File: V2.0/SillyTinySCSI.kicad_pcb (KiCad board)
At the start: 4 copper layers, 53.5 x 25 mm, 48 parts, among them J1 DB25_Plug, J2 Micro_SD_Card_Det1, U1 74LVT125, U2 74LVT245, U3 74LVT125, U4 74LVT245, U5 TLV75728PDBVR, U6 Pico W

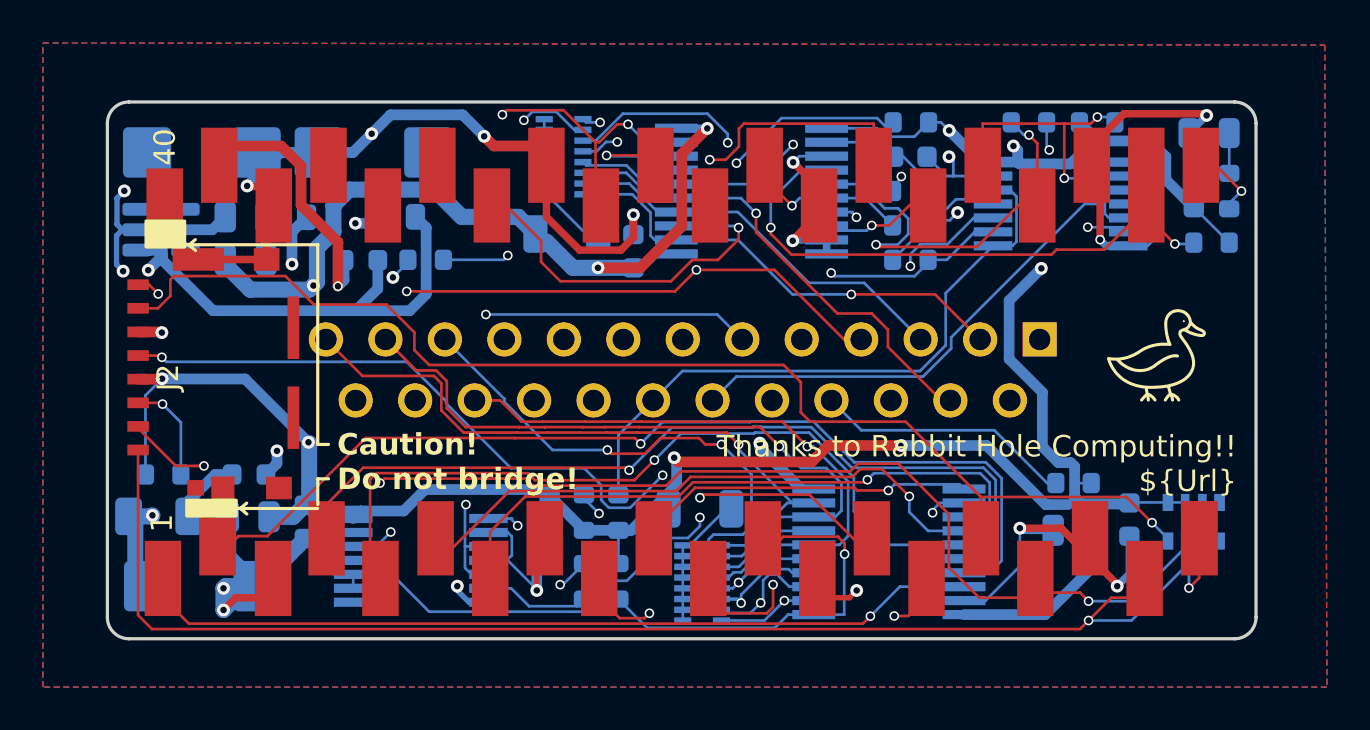
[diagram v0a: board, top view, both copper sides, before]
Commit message: before ar
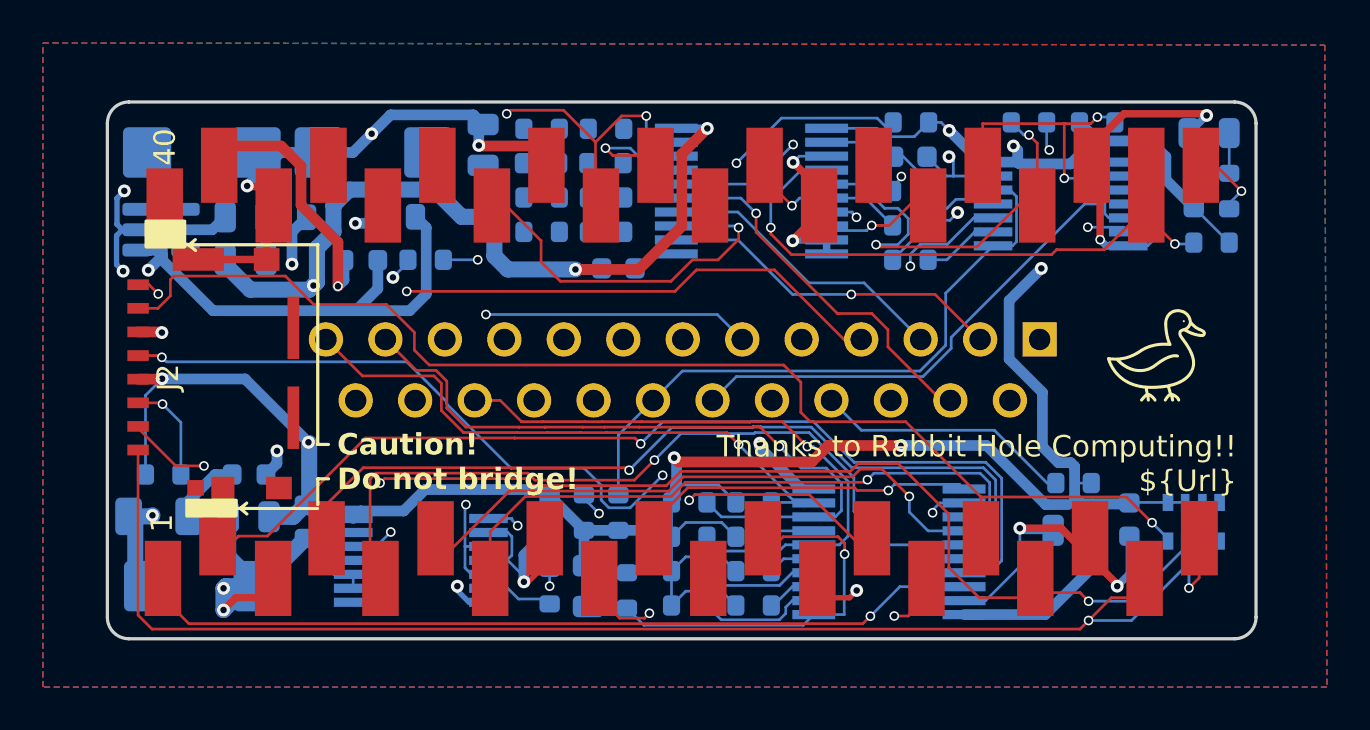
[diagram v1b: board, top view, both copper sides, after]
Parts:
- removed RN1, RN2: 100, Resistor_SMD:R_Array_Convex_8x0602
- added C14: 10uF, Capacitor_SMD:C_0805_2012Metric, B.Cu at (130.4, 72.8)
- added C15: 10uF, Capacitor_SMD:C_0805_2012Metric, B.Cu at (125.5, 52.2)
- added R14: 110, Resistor_SMD:R_0603_1608Metric, B.Cu at (128.2, 51.5)
- added R21: 110, Resistor_SMD:R_0603_1608Metric, B.Cu at (131.2, 51.5)
- added R22: 110, Resistor_SMD:R_0603_1608Metric, B.Cu at (128.2, 53.1)
- added R23: 110, Resistor_SMD:R_0603_1608Metric, B.Cu at (131.2, 53.1)
- added R24: 110, Resistor_SMD:R_0603_1608Metric, B.Cu at (135.1, 73.7)
- added R25: 110, Resistor_SMD:R_0603_1608Metric, B.Cu at (138.1, 73.7)
- added R26: 110, Resistor_SMD:R_0603_1608Metric, B.Cu at (135.1, 72.1)
- added R27: 110, Resistor_SMD:R_0603_1608Metric, B.Cu at (138.1, 72.1)
- added R28: 110, Resistor_SMD:R_0603_1608Metric, B.Cu at (135.1, 70.5)
- added R29: 110, Resistor_SMD:R_0603_1608Metric, B.Cu at (138.1, 70.5)
- added R3: 110, Resistor_SMD:R_0603_1608Metric, B.Cu at (128.2, 56.3)
- added R30: 110, Resistor_SMD:R_0603_1608Metric, B.Cu at (135.1, 68.9)
- added R31: 110, Resistor_SMD:R_0603_1608Metric, B.Cu at (138.1, 68.9)
- added R8: 110, Resistor_SMD:R_0603_1608Metric, B.Cu at (131.2, 56.3)
- R10, R11: value 10 -> 110; footprint Resistor_SMD:R_1206_3216Metric -> Resistor_SMD:R_0603_1608Metric
- moved R10 16.3 mm to (128.2, 54.7), turned to 180 degrees
- moved R11 2.49 mm to (131.2, 54.7), turned to 180 degrees
- moved R1 1.62 mm to (128.6, 72.8)
- moved C1 1.06 mm to (131.8, 58.0), turned to 0 degrees
- moved R6 0.58 mm to (132.2, 73.0)
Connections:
- R10 pad 1: +2V8 -> ~{SCSI_CD}
- R10 pad 2: Net-(RN1-R1.2) -> +2V8
- R11 pad 1: +2V8 -> ~{SCSI_REQ}
- R11 pad 2: Net-(RN2-R1.2) -> +2V8
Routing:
- net ~{IN_RST}: track 47.8 -> 0.00 mm, vias 2 -> 0
- net ~{SCSI_DB5}: track 28.7 -> 2.09 mm, vias 2 -> 0
- net +2V8: track 194.6 -> 220.0 mm
- net ~{GPIO_DBP}: track 27.5 -> 3.56 mm, vias 2 -> 0
- net ~{SCSI_DB3}: track 22.5 -> 2.21 mm, vias 1 -> 0
- net ~{SCSI_DB1}: track 19.0 -> 2.34 mm, vias 1 -> 0
- net ~{SCSI_SEL}: track 41.6 -> 25.6 mm, vias 1 -> 0
- net ~{SCSI_DB2}: track 19.8 -> 5.50 mm, vias 1 -> 0
- net ~{SCSI_DB0}: track 20.1 -> 5.79 mm, vias 1 -> 0
- net ~{SCSI_BSY}: track 39.7 -> 26.7 mm, vias 3 -> 2
- net ~{SCSI_ACK}: track 26.2 -> 13.9 mm, vias 2 -> 1
- net GND: track 131.8 -> 121.6 mm, vias 22 -> 21
- net ~{SCSI_RST}: track 45.9 -> 36.6 mm, vias 4 -> 2
- net Net-(RN2-R1.2): track 6.58 -> 0.00 mm
- net Net-(RN1-R1.2): track 5.90 -> 0.00 mm
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
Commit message: before ar2
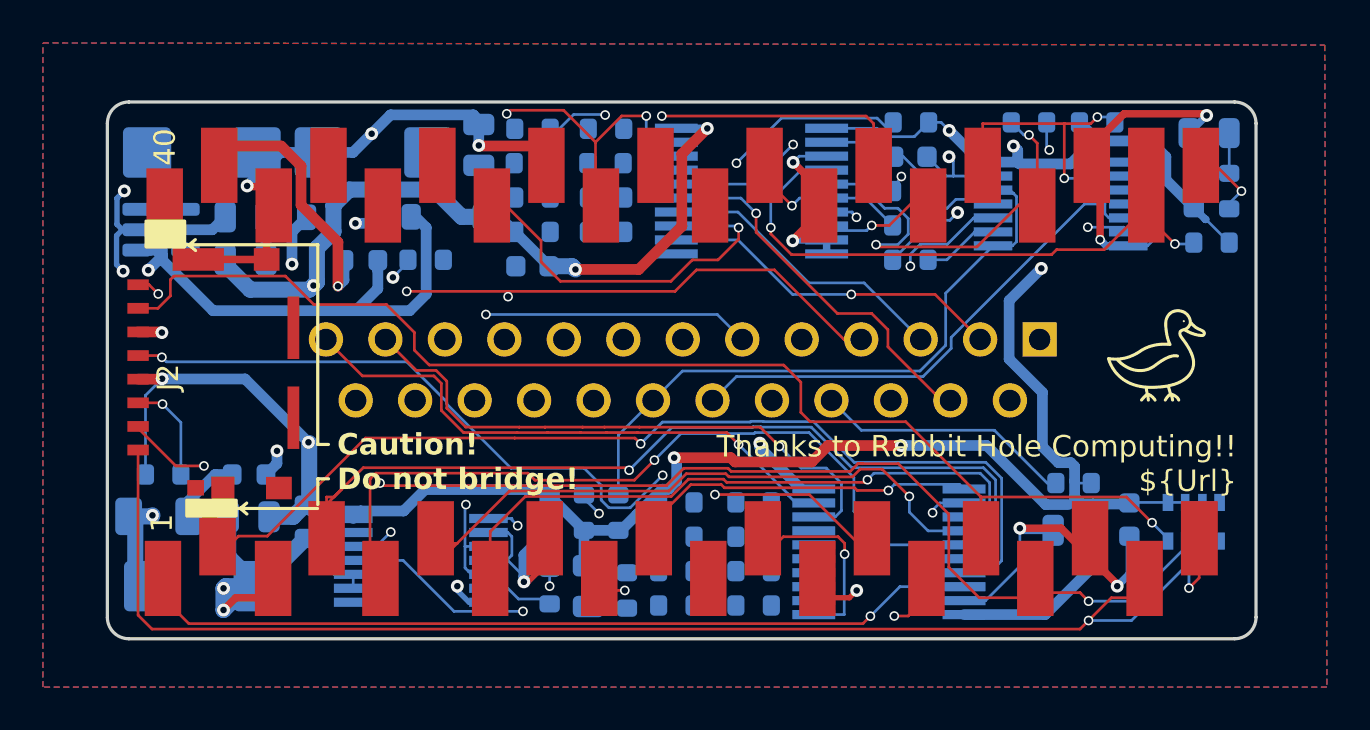
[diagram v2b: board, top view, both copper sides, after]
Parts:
- moved C1 4.00 mm to (127.8, 57.9), turned to 180 degrees
- moved R24 0.60 mm to (134.5, 73.7)
- moved R26 0.60 mm to (134.5, 72.1)
- moved R28 0.60 mm to (134.5, 70.5)
- moved R30 0.60 mm to (134.5, 68.9)
- moved R10 0.42 mm to (127.8, 54.7)
- moved R14 0.42 mm to (127.8, 51.5)
- moved R3 0.42 mm to (127.8, 56.3)
- moved R22 0.42 mm to (127.8, 53.1)
- moved C15 0.20 mm to (125.3, 52.2)
- moved D2 0.20 mm to (123.8, 55.6)
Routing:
- net ~{IN_RST}: track 0.00 -> 48.0 mm, vias 0 -> 2
- net ~{SCSI_DB4}: track 28.6 -> 0.00 mm, vias 1 -> 0
- net +2V8: track 220.0 -> 197.9 mm
- net ~{GPIO_ACK}: track 15.7 -> 0.00 mm, vias 2 -> 0
- net ~{SCSI_RST}: track 36.6 -> 49.9 mm, vias 2 -> 4
- net ~{DATA_DIR}: track 37.5 -> 28.3 mm
- net ~{SCSI_DB0}: track 5.79 -> 0.00 mm
- net ~{SCSI_DB2}: track 5.50 -> 0.00 mm
- net ~{SCSI_DB6}: track 32.7 -> 27.4 mm
- net ~{GPIO_DB2}: track 38.8 -> 42.4 mm
- net ~{SCSI_DB7}: track 28.6 -> 25.8 mm
- net ~{SCSI_DB1}: track 2.34 -> 0.00 mm
- net ~{SCSI_DB3}: track 2.21 -> 0.00 mm
- net ~{SCSI_DB5}: track 2.09 -> 0.00 mm
- net GND: track 121.6 -> 120.2 mm
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
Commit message: ar2, re-route
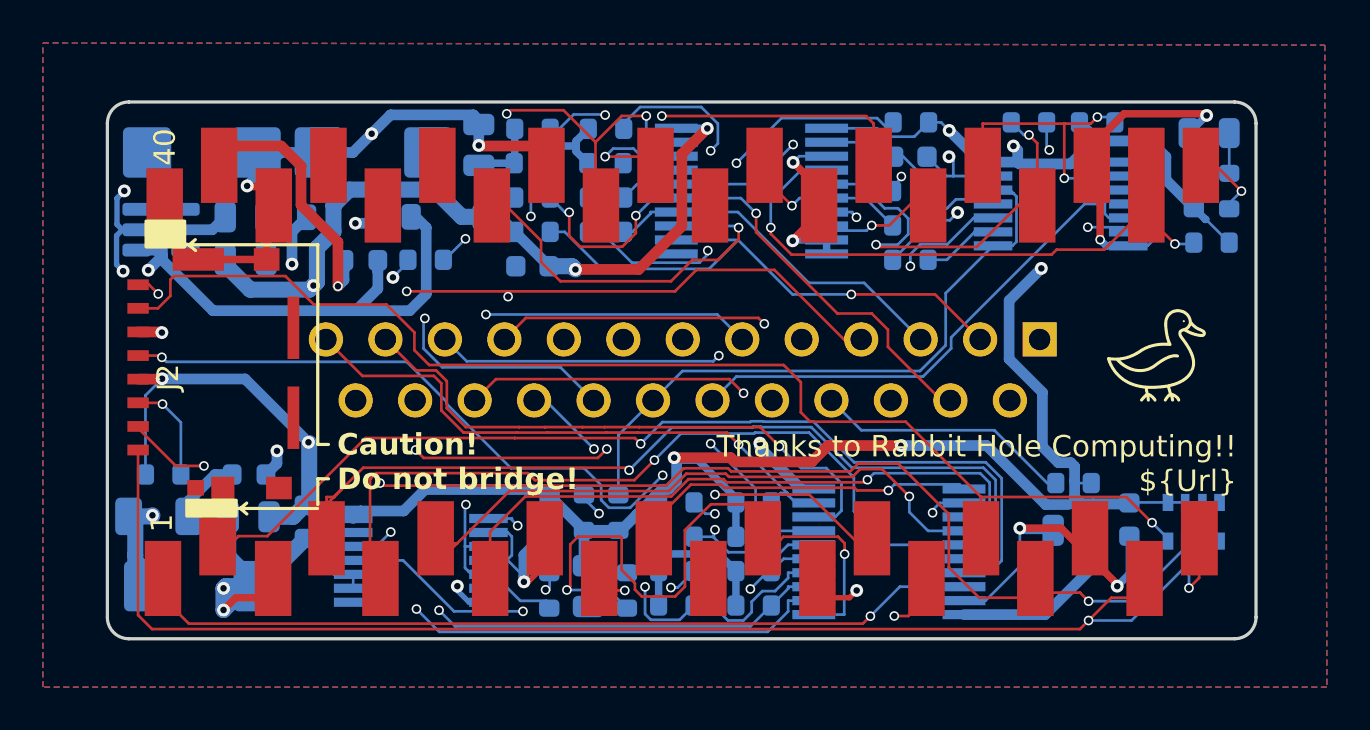
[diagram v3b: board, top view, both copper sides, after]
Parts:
- moved R1 0.20 mm to (128.6, 73.0)
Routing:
- net ~{SCSI_DB0}: track 0.00 -> 54.8 mm, vias 0 -> 4
- net ~{SCSI_DB1}: track 0.00 -> 42.9 mm, vias 0 -> 2
- net +2V8: track 197.9 -> 228.5 mm
- net ~{SCSI_DB3}: track 0.00 -> 30.0 mm, vias 0 -> 2
- net ~{SCSI_DB4}: track 0.00 -> 28.5 mm, vias 0 -> 2
- net ~{SCSI_DB5}: track 0.00 -> 25.7 mm, vias 0 -> 2
- net ~{DATA_DIR}: track 28.3 -> 50.3 mm, vias 2 -> 3
- net ~{SCSI_DB2}: track 0.00 -> 21.2 mm, vias 0 -> 2
- net ~{SCSI_SEL}: track 25.6 -> 41.8 mm, vias 0 -> 1
- net ~{GPIO_ACK}: track 0.00 -> 15.7 mm, vias 0 -> 2
- net ~{SCSI_ACK}: track 14.0 -> 24.9 mm, vias 1 -> 2
- net ~{SCSI_MSG}: track 16.1 -> 26.1 mm
- net ~{SCSI_CD}: track 17.2 -> 26.6 mm, vias 1 -> 3
- net ~{SCSI_BSY}: track 27.5 -> 35.9 mm, vias 2 -> 3
- net ~{SCSI_DB6}: track 27.4 -> 33.0 mm, vias 1 -> 2
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
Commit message: ar3 all but pwr
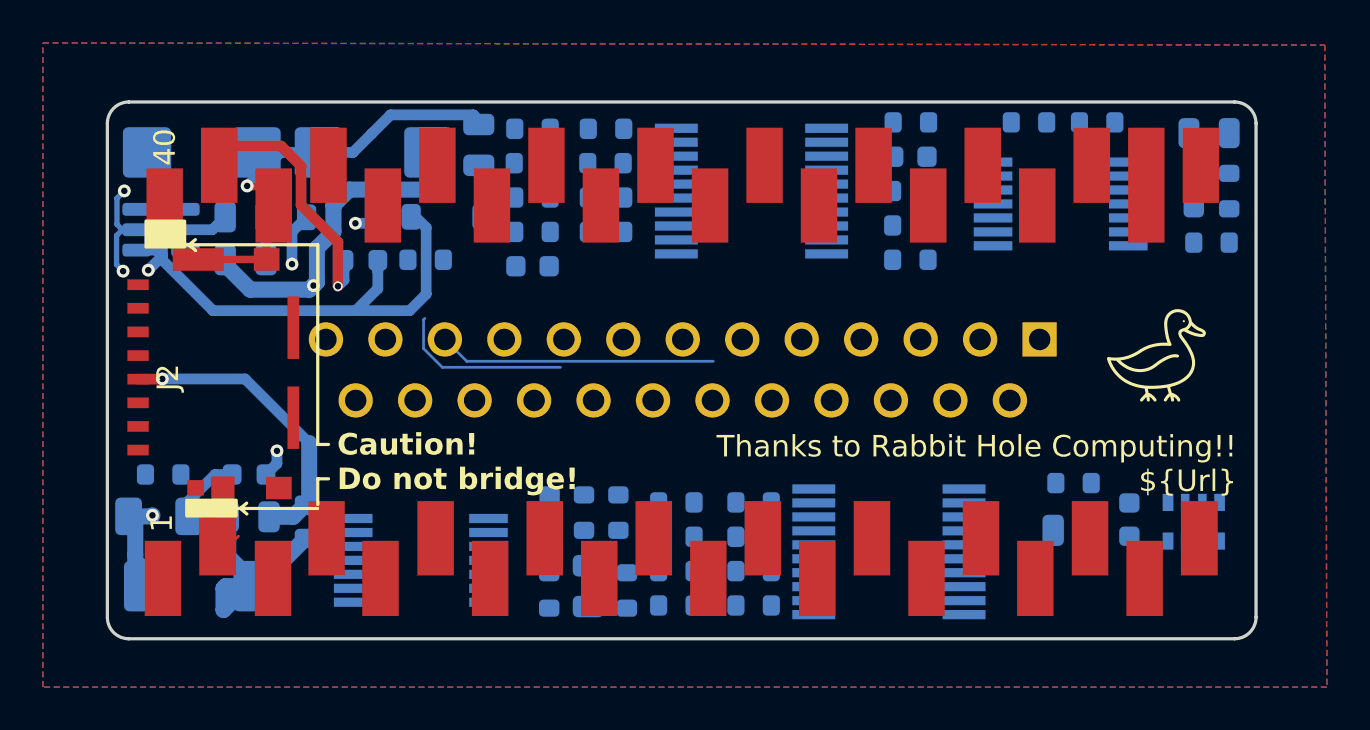
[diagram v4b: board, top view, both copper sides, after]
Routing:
- net +2V8: track 228.5 -> 41.0 mm, vias 10 -> 2
- net GND: track 120.2 -> 41.9 mm, vias 21 -> 3
- net /cpu/SDIO_D2: track 62.5 -> 0.00 mm, vias 1 -> 0
- net /cpu/SDIO_D1: track 60.3 -> 0.00 mm, vias 3 -> 0
- net /cpu/SDIO_D3: track 58.5 -> 0.00 mm, vias 2 -> 0
- net /cpu/SDIO_D0: track 58.3 -> 0.00 mm, vias 1 -> 0
- net ~{SCSI_DB0}: track 54.8 -> 0.00 mm, vias 4 -> 0
- net ~{DATA_DIR}: track 50.3 -> 0.00 mm, vias 3 -> 0
- net ~{SCSI_RST}: track 50.3 -> 0.00 mm, vias 4 -> 0
- net ~{IN_RST}: track 48.2 -> 0.00 mm, vias 2 -> 0
- net /cpu/SDIO_CMD: track 46.6 -> 0.00 mm, vias 2 -> 0
- net ~{GPIO_DB1}: track 46.3 -> 1.39 mm, vias 1 -> 0
- net ~{OUT_BSY}: track 42.1 -> 0.00 mm, vias 4 -> 0
- net ~{SCSI_SEL}: track 41.8 -> 0.00 mm, vias 1 -> 0
- net ~{GPIO_DB2}: track 42.4 -> 2.46 mm, vias 1 -> 0
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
